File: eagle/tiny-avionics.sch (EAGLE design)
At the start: 69 parts, among them IC1 BQ24022, J1 USB-MICROB, J3 JST-PH-2-SMT-RA, U1 LP5907, U2 M25P10-AVMN6TP_TR, U3 LSM9DS0, U5 LTC1998, U6 ATMEGA32U4-AU, X1 8MHz

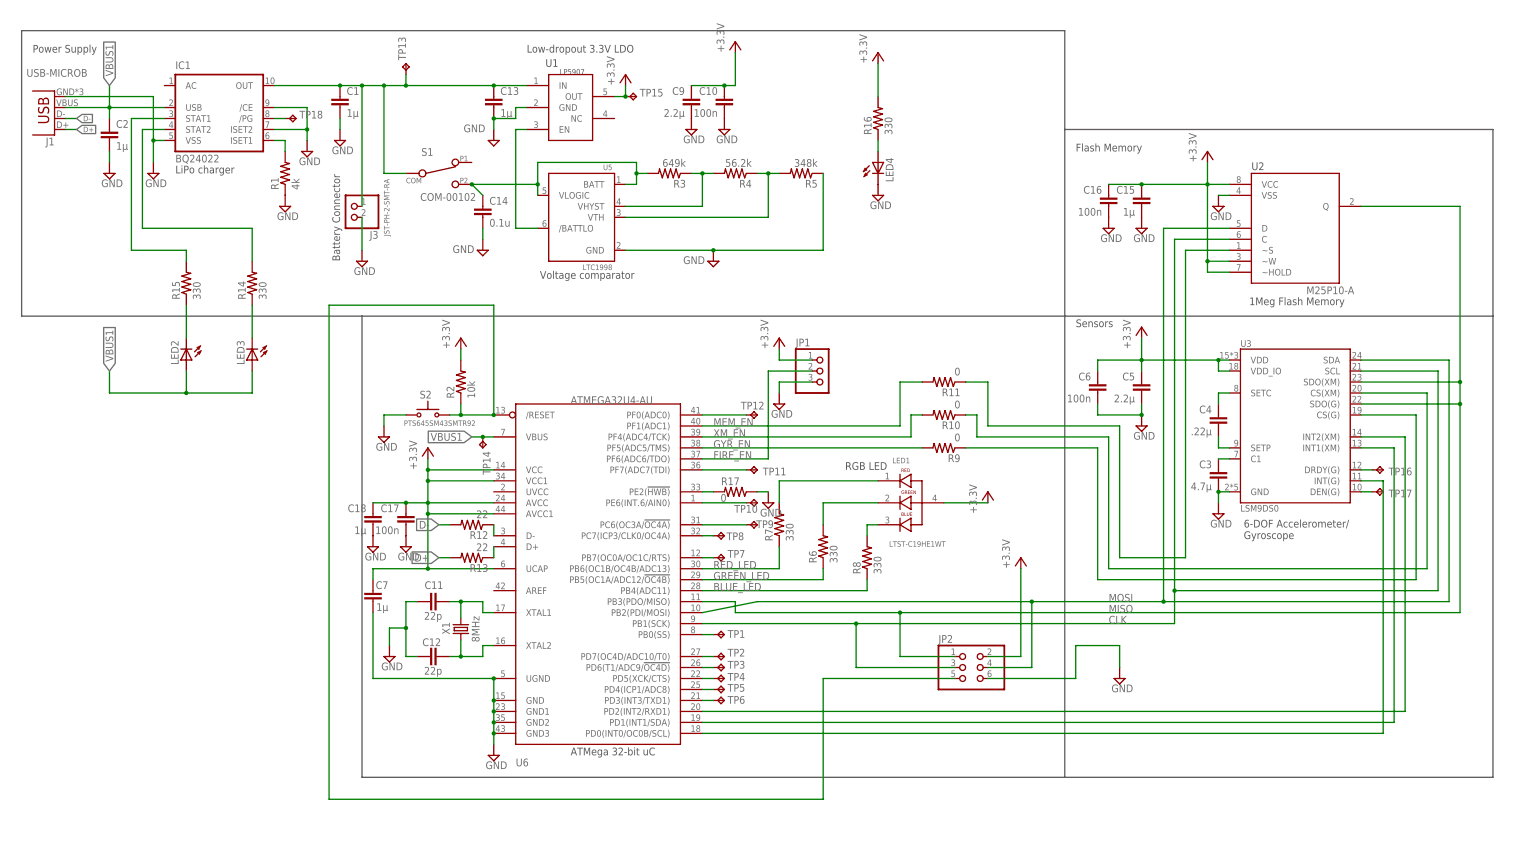
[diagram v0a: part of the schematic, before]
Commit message: Merge commit to overwrite eagle files
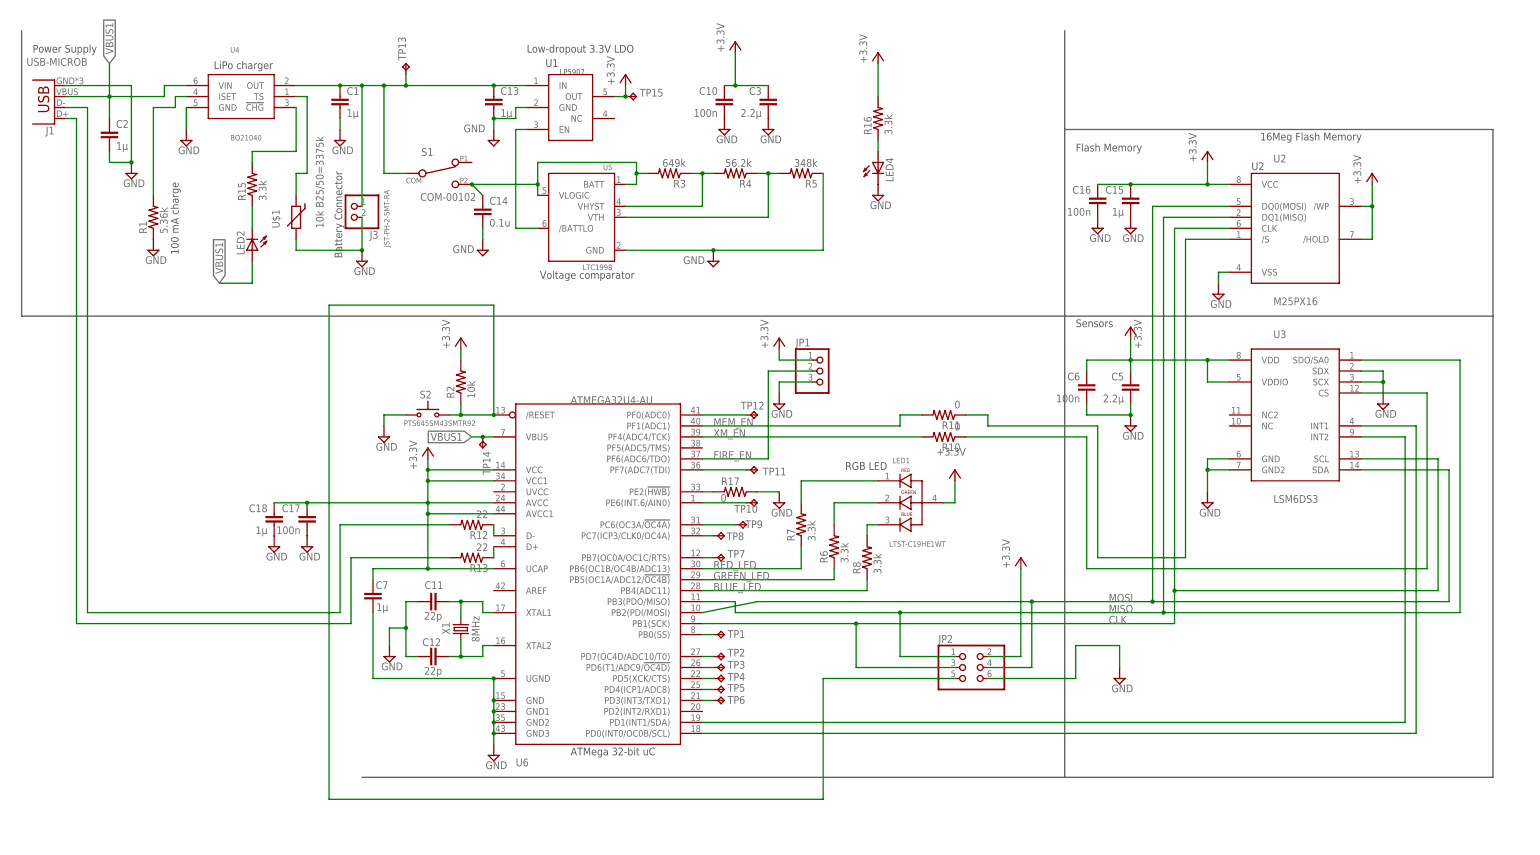
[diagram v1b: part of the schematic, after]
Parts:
- removed C4: .22µ, rcl:C-EUC0603
- removed C9: 2.2µ, rcl:C-EUC0603
- removed IC1: BQ24022, tinyav-lib:BQ24022
- removed LED3: (no value), adafruit:LEDCHIP-LED0603
- removed R14: 330, rcl:R-US_R0805
- removed R9: 0, rcl:R-US_R0603
- removed TP16, TP17, TP18: TPTP08R, testpad:TPTP08R
- added U$1: 10k B25/50=3375k, tinyav-lib:THERMISTOR-SMD0603
- added U4: BQ21040, tinyav-lib:BQ21040
- C2: device rcl:C-EUC0805 -> rcl:C-EUC0603
- C3: value 4.7µ -> 2.2µ
- R1: value 4k -> 5.36k
- R15, R16, R6, R7, R8: value 330 -> 3.3k; device rcl:R-US_R0805 -> rcl:R-US_R0603
- R2: device rcl:R-US_R0805 -> rcl:R-US_R0603
- U2: value M25P10-AVMN6TP_TR -> M25PX16; device SOIC127P600X175-8N:M25P10-AVMN6TP_TR -> tinyav-lib:M25PX16
- U3: value LSM9DS0 -> LSM6DS3; device LSM9DS0:LSM9DS0 -> tinyav-lib:LSM6DS3
- X1: device IQD-Frequency-Products:CRYSTALS-NOGND-HC49/4H -> tinyav-lib:CRYSTAL-NOGND-SMD
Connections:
- net N$52 renamed TP3
- net N$54 renamed TP12
- net N$55 renamed TP11
- net N$56 renamed TP10
- net N$57 renamed TP9
- net N$58 renamed TP8
- net N$59 renamed TP7
- net N$60 renamed TP1
- net N$61 renamed TP2
- net N$62 renamed TP4
- net N$63 renamed TP5
- net N$64 renamed TP6
- removed net GYR_EN: R9.1, U3.CS(G)
- removed net N$16: U3.INT2(XM), U6.PD2(INT2/RXD1)
- removed net N$17: U3.INT1(XM), U6.PD1(INT1/SDA)
- removed net N$19: U3.INT(G), U6.PD0(INT0/OC0B/SCL)
- removed net N$20: R9.2, U6.PF5(ADC5/TMS)
- removed net N$50: IC1G$1.STAT1, R15.2
- removed net N$51: IC1G$1.STAT2, R14.2
- removed net N$66: TP17.TP, U3.DEN(G)
- removed net N$67: TP16.TP, U3.DRDY(G)
- removed net N$68: IC1G$1./PG, TP18.TP
- net CLK: now also U2.CLK; no longer U2.C
- net GND: now also C3.2, U$1.2, U3.GND2, U3.SCX, U3.SDX, U4.GND; no longer C3.1, C9.2, IC1G$1./CE, IC1G$1.ISET2, IC1G$1.VSS
- net MEM_EN: now also U2./S; no longer U2.~S
- net MISO: now also U2.DQ1(MISO), U3.SDO/SA0; no longer U2.Q, U3.SDO(G), U3.SDO(XM)
- net MOSI: now also U2.DQ0(MOSI); no longer U2.D
- net N$10: now also U3.INT1, U6.PD0(INT0/OC0B/SCL); no longer C4.2, U3.SETC
- net N$11: now also U3.INT2, U6.PD1(INT1/SDA); no longer C4.1, U3.SETP
- net N$13: now also U4.OUT; no longer IC1G$1.OUT
- net N$4: now also R15.2, U4.!CHG; no longer IC1G$1.ISET1, R1.2
- net N$49: now also R1.2, U4.ISET; no longer LED3.C, R14.1
- net N$9: now also U$1.1, U4.TS; no longer C3.2, U3.C1
- net VBUS1: now also U4.VIN; no longer IC1G$1.USB, LED3.A
- net VCC: now also C3.1, U2./HOLD, U2./WP, U3.VDDIO; no longer C9.1, U2.~HOLD, U2.~W, U3.VDD_IO
- net XM_EN: now also U3.CS; no longer U3.CS(XM)
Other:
- note added: "100 mA charge"
- note added: "16Meg Flash Memory"
- note removed: "1Meg Flash Memory"
- note removed: "6-DOF Accelerometer/ Gyroscope"
- moved on the sheet: C15, C16, C17, C18, C3, C5, C6, J1, LED2, R1, R10, R11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
